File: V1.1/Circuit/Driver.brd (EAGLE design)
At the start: 61.6 x 54.6 mm, 32 parts, among them IC1 DRV8300DIPWR, IC2 CD74HC4049PWR, U1 INA240A1PWR, U2 INA240A1PWR, U3 INA240A1PWR

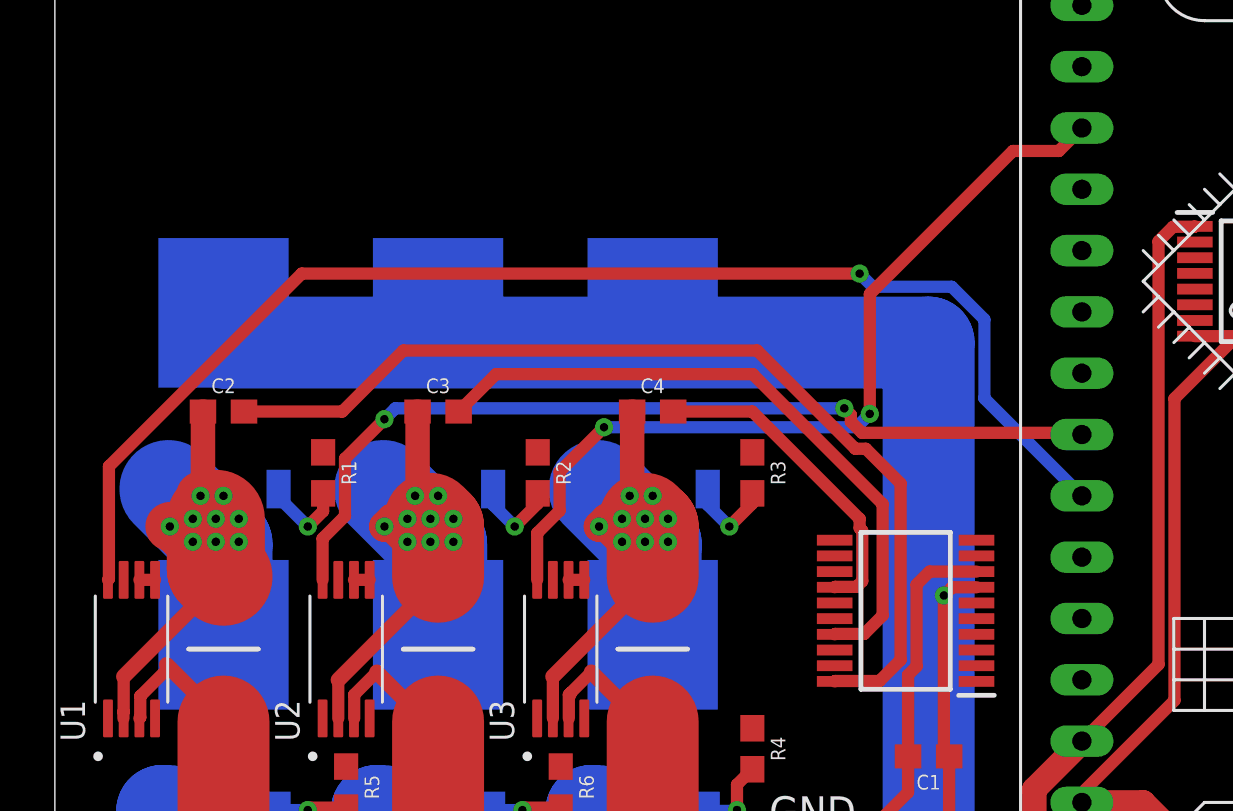
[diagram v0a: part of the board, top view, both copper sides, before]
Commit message: Ready for autoroutering 5
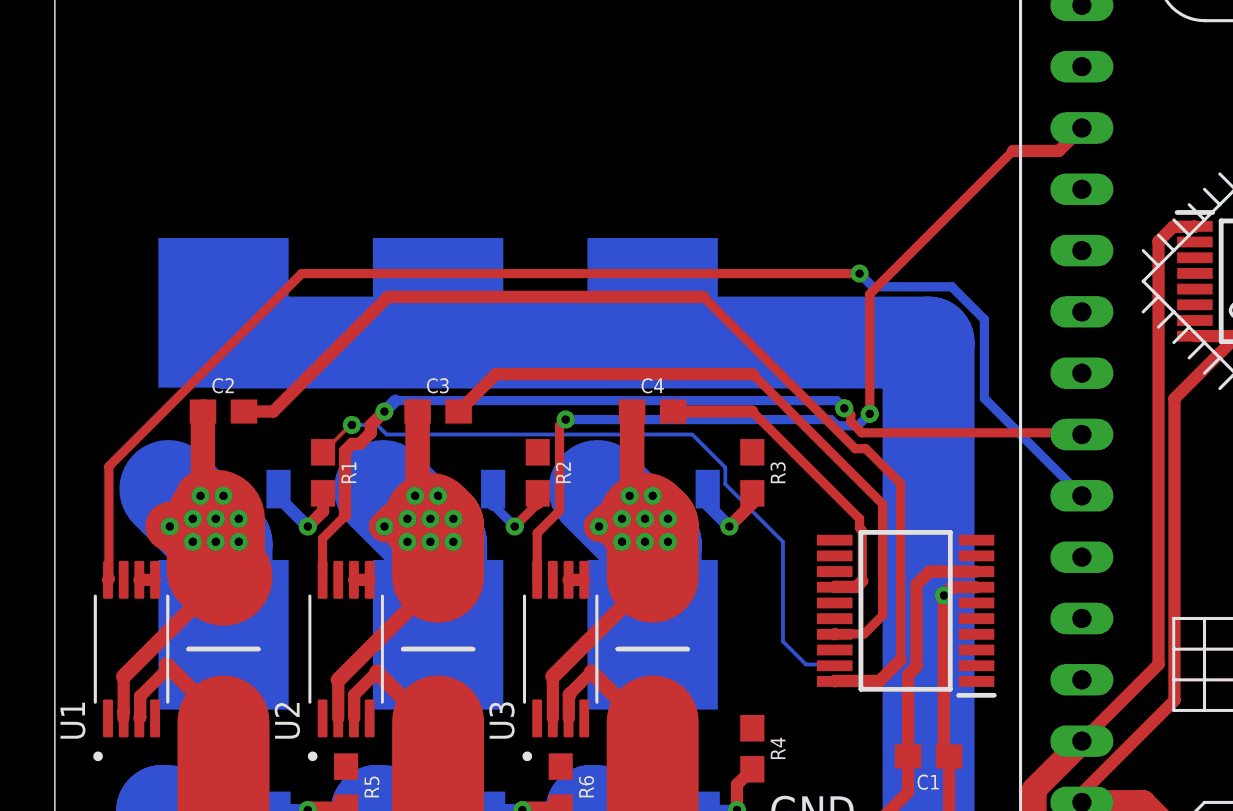
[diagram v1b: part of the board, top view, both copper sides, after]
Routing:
- net GHA: track 0.00 -> 28.7 mm, vias 0 -> 1
- net BSTA: track 40.9 -> 42.8 mm
- net PA3: track 35.3 -> 36.6 mm
- net PB0: track 37.4 -> 38.0 mm
